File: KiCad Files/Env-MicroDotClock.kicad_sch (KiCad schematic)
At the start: 40 parts, among them IC1 IS31FL3730-QFLS2-TR, IC2 IS31FL3730-QFLS2-TR, IC3 IS31FL3730-QFLS2-TR, IC4 IS31FL3730-QFLS2-TR, M1 LTP-305G, M2 LTP-305G, M3 LTP-305G, M4 LTP-305G, M5 LTP-305G, M6 LTP-305G, M7 LTP-305G, M8 LTP-305G, Q1 2SC1815, SW1 SW_Push, SW2 SW_Push, SW3 SW_Push, SW4 SW_Push, SW5 DIP SPST, U1 Pico, U3 DS3231M

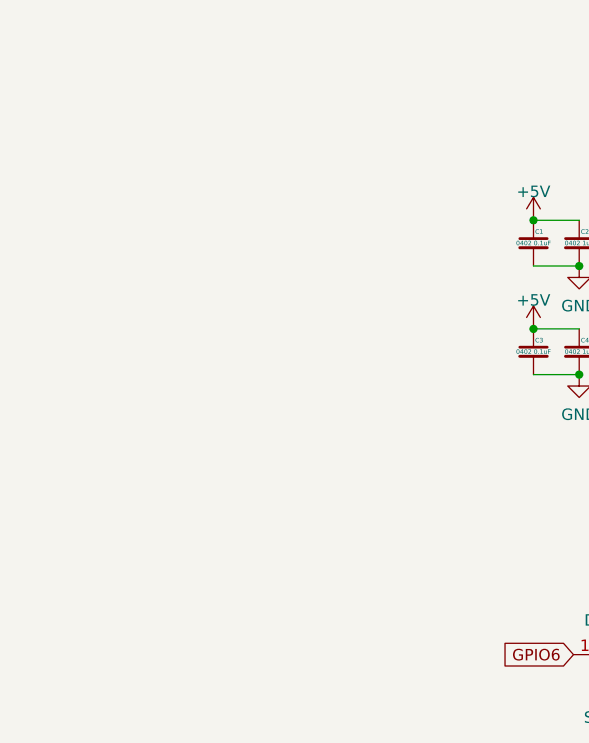
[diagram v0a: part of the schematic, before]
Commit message: dont recall what I changed, probably cleaned some bits up before generating gerber
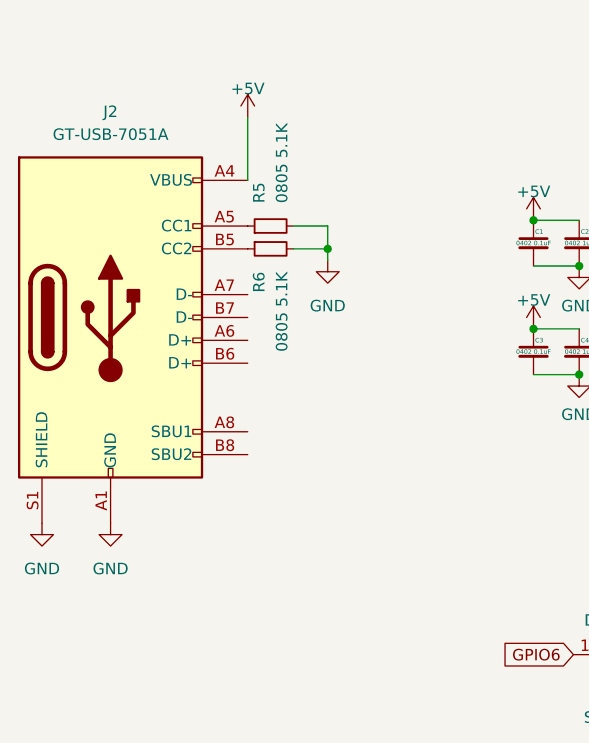
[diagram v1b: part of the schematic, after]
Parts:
- added J2: GT-USB-7051A, Connector_USB:USB_C_Receptacle_G-Switch_GT-USB-7051x, symbol Connector:USB_C_Receptacle_USB2.0
- added R5, R6: 0805 5.1K, Resistor_SMD:R_0805_2012Metric, symbol Device:R_Small
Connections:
- net +5V: now also J2.A4 (VBUS), J2.A9 (VBUS), J2.B4 (VBUS), J2.B9 (VBUS)
- net GND: now also J2.A1 (GND), J2.A12 (GND), J2.B1 (GND), J2.B12 (GND), J2.S1 (SHIELD), R5.2, R6.2
- new net: J2.B5 (CC2), R6.1
- new net: J2.A5 (CC1), R5.1
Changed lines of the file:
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@@
   (junction (at 163.195 168.91) (diameter 0) (color 0 0 0 0)
   )
+  (junction (at -4.445 36.83) (diameter 0) (color 0 0 0 0)
+  )
   (junction (at 170.18 129.54) (diameter 0) (color 0 0 0 0)
   )
@@
     (stroke (width 0) (type default))
   )
+  (wire (pts (xy -4.445 38.1) (xy -4.445 36.83))
+    (stroke (width 0) (type default))
+  )
   (wire (pts (xy 173.355 49.53) (xy 173.355 36.83))
     (stroke (width 0) (type default))
@@
     (stroke (width 0) (type default))
   )
+  (wire (pts (xy -8.255 34.29) (xy -4.445 34.29))
+    (stroke (width 0) (type default))
+  )
   (wire (pts (xy 33.02 81.915) (xy 33.02 94.615))
     (stroke (width 0) (type default))
@@
     (stroke (width 0) (type default))
   )
+  (wire (pts (xy -4.445 34.29) (xy -4.445 36.83))
+    (stroke (width 0) (type default))
+  )
   (wire (pts (xy 33.02 94.615) (xy 33.02 105.41))
     (stroke (width 0) (type default))
@@
     (stroke (width 0) (type default))
   )
+  (wire (pts (xy -13.335 22.225) (xy -13.335 29.21))
+    (stroke (width 0) (type default))
+  )
+  (wire (pts (xy -4.445 36.83) (xy -8.255 36.83))
+    (stroke (width 0) (type default))
+  )
   (wire (pts (xy 99.06 158.75) (xy 99.06 162.56))
     (stroke (width 0) (type default))
@@
     )
   )
+  (symbol (lib_id "Device:R_Small") (at -10.795 36.83 90) (mirror x) (unit 1)
+    (in_bom yes) (on_board yes) (dnp no)
+    (property "Reference" "R6" (at -12.065 39.37 0)
+      (effects (font (size 1.27 1.27)) (justify left))
+    )
+    (property "Value" "0805 5.1K" (at -9.525 39.37 0)
+      (effects (font (size 1.27 1.27)) (justify left))
+    )
+    (property "Footprint" "Resistor_SMD:R_0805_2012Metric" (at -10.795 36.83 0)
+      (effects (font (size 1.27 1.27)) hide)
+    )
+    (property "Datasheet" "~" (at -10.795 36.83 0)
+      (effects (font (size 1.27 1.27)) hide)
+    )
+    (pin "1")
+    (pin "2")
+    (instances
+      (project "Env-MicroDotClock"
+        (path "/3dbeb8d8-208e-4f6d-8d30-b14372f68a4f"
+          (reference "R6") (unit 1)
+        )
+      )
+    )
+  )
   (symbol (lib_id "power:GND") (at 80.645 73.025 0) (mirror y) (unit 1)
     (in_bom yes) (on_board yes) (dnp no) (fields_autoplaced)
@@
     )
   )
+  (symbol (lib_id "Connector:USB_C_Receptacle_USB2.0") (at -28.575 44.45 0) (unit 1)
+    (in_bom yes) (on_board yes) (dnp no) (fields_autoplaced)
+    (property "Reference" "J2" (at -28.575 21.59 0)
+      (effects (font (size 1.27 1.27)))
+    )
+    (property "Value" "GT-USB-7051A" (at -28.575 24.13 0)
+      (effects (font (size 1.27 1.27)))
+    )
+    (property "Footprint" "Connector_USB:USB_C_Receptacle_G-Switch_GT-USB-7051x" (at -24.765 44.45 0)
+      (effects (font (size 1.27 1.27)) hide)
+    )
+    (property "Datasheet" "https://www.usb.org/sites/default/files/documents/usb_type-c.zip" (at -24.765 44.45 0)
+      (effects (font (size 1.27 1.27)) hide)
+    )
+    (pin "A1")
+    (pin "A12")
+    (pin "A4")
+    (pin "A5")
+    (pin "A6")
+    (pin "A7")
+    (pin "A8")
+    (pin "A9")
+    (pin "B1")
+    (pin "B12")
+    (pin "B4")
+    (pin "B5")
+    (pin "B6")
+    (pin "B7")
+    (pin "B8")
+    (pin "B9")
+    (pin "S1")
+    (instances
+      (project "Env-MicroDotClock"
+        (path "/3dbeb8d8-208e-4f6d-8d30-b14372f68a4f"
+          (reference "J2") (unit 1)
+        )
+      )
+    )
+  )
   (symbol (lib_id "Transistor_BJT:BC817") (at 154.305 181.61 0) (unit 1)
     (in_bom yes) (on_board yes) (dnp no) (fields_autoplaced)
@@
     )
   )
+  (symbol (lib_id "power:+5V") (at -13.335 22.225 0) (unit 1)
+    (in_bom yes) (on_board yes) (dnp no) (fields_autoplaced)
+    (property "Reference" "#PWR044" (at -13.335 26.035 0)
+      (effects (font (size 1.27 1.27)) hide)
+    )
+    (property "Value" "+5V" (at -13.335 19.05 0)
+      (effects (font (size 1.27 1.27)))
+    )
+    (property "Footprint" "" (at -13.335 22.225 0)
+      (effects (font (size 1.27 1.27)) hide)
+    )
+    (property "Datasheet" "" (at -13.335 22.225 0)
+      (effects (font (size 1.27 1.27)) hide)
+    )
+    (pin "1")
+    (instances
+      (project "Env-MicroDotClock"
+        (path "/3dbeb8d8-208e-4f6d-8d30-b14372f68a4f"
+          (reference "#PWR044") (unit 1)
+        )
+      )
+    )
+  )
   (symbol (lib_id "ltp-305g:LTP-305G") (at 102.87 104.775 0) (unit 1)
     (in_bom yes) (on_board yes) (dnp no) (fields_autoplaced)
@@
     )
   )
+  (symbol (lib_id "power:GND") (at -28.575 67.31 0) (mirror y) (unit 1)
+    (in_bom yes) (on_board yes) (dnp no) (fields_autoplaced)
+    (property "Reference" "#PWR046" (at -28.575 73.66 0)
+      (effects (font (size 1.27 1.27)) hide)
+    )
+    (property "Value" "GND" (at -28.575 72.39 0)
+      (effects (font (size 1.27 1.27)))
+    )
+    (property "Footprint" "" (at -28.575 67.31 0)
+      (effects (font (size 1.27 1.27)) hide)
+    )
+    (property "Datasheet" "" (at -28.575 67.31 0)
+      (effects (font (size 1.27 1.27)) hide)
+    )
+    (pin "1")
+    (instances
+      (project "Env-MicroDotClock"
+        (path "/3dbeb8d8-208e-4f6d-8d30-b14372f68a4f"
+          (reference "#PWR046") (unit 1)
+        )
+      )
+    )
+  )
   (symbol (lib_id "ltp-305g:LTP-305G") (at 229.87 34.925 0) (unit 1)
     (in_bom yes) (on_board yes) (dnp no) (fields_autoplaced)
@@
     )
   )
+  (symbol (lib_id "Device:R_Small") (at -10.795 34.29 90) (unit 1)
+    (in_bom yes) (on_board yes) (dnp no)
+    (property "Reference" "R5" (at -12.065 31.75 0)
+      (effects (font (size 1.27 1.27)) (justify left))
+    )
+    (property "Value" "0805 5.1K" (at -9.525 31.75 0)
+      (effects (font (size 1.27 1.27)) (justify left))
+    )
+    (property "Footprint" "Resistor_SMD:R_0805_2012Metric" (at -10.795 34.29 0)
+      (effects (font (size 1.27 1.27)) hide)
+    )
+    (property "Datasheet" "~" (at -10.795 34.29 0)
+      (effects (font (size 1.27 1.27)) hide)
+    )
+    (pin "1")
+    (pin "2")
+    (instances
+      (project "Env-MicroDotClock"
+        (path "/3dbeb8d8-208e-4f6d-8d30-b14372f68a4f"
+          (reference "R5") (unit 1)
+        )
+      )
+    )
+  )
   (symbol (lib_id "power:GND") (at 23.495 38.735 0) (unit 1)
     (in_bom yes) (on_board yes) (dnp no) (fields_autoplaced)
@@
     )
   )
+  (symbol (lib_id "power:GND") (at -4.445 38.1 0) (mirror y) (unit 1)
+    (in_bom yes) (on_board yes) (dnp no) (fields_autoplaced)
+    (property "Reference" "#PWR047" (at -4.445 44.45 0)
+      (effects (font (size 1.27 1.27)) hide)
+    )
+    (property "Value" "GND" (at -4.445 43.18 0)
+      (effects (font (size 1.27 1.27)))
+    )
+    (property "Footprint" "" (at -4.445 38.1 0)
+      (effects (font (size 1.27 1.27)) hide)
+    )
+    (property "Datasheet" "" (at -4.445 38.1 0)
+      (effects (font (size 1.27 1.27)) hide)
+    )
+    (pin "1")
+    (instances
+      (project "Env-MicroDotClock"
+        (path "/3dbeb8d8-208e-4f6d-8d30-b14372f68a4f"
+          (reference "#PWR047") (unit 1)
+        )
+      )
+    )
+  )
   (symbol (lib_id "power:+5V") (at 18.415 33.655 0) (unit 1)
     (in_bom yes) (on_board yes) (dnp no) (fields_autoplaced)
@@
         )
       )
+    )
+  )
+  (symbol (lib_id "power:GND") (at -36.195 67.31 0) (mirror y) (unit 1)
+    (in_bom yes) (on_board yes) (dnp no) (fields_autoplaced)
+    (property "Reference" "#PWR045" (at -36.195 73.66 0)
+      (effects (font (size 1.27 1.27)) hide)
+    )
+    (property "Value" "GND" (at -36.195 72.39 0)
+      (effects (font (size 1.27 1.27)))
+    )
+    (property "Footprint" "" (at -36.195 67.31 0)
+      (effects (font (size 1.27 1.27)) hide)
+    )
+    (property "Datasheet" "" (at -36.195 67.31 0)
+      (effects (font (size 1.27 1.27)) hide)
+    )
+    (pin "1")
+    (instances
+      (project "Env-MicroDotClock"
+        (path "/3dbeb8d8-208e-4f6d-8d30-b14372f68a4f"
+          (reference "#PWR045") (unit 1)
+        )
+      )

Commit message: updated to reflect current vision.
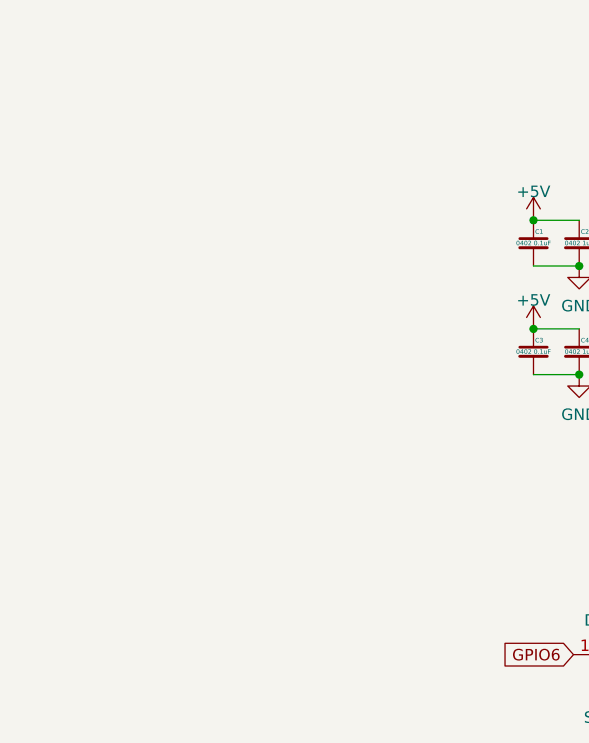
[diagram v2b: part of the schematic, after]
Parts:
- removed J2: GT-USB-7051A, Connector_USB:USB_C_Receptacle_G-Switch_GT-USB-7051x, symbol Connector:USB_C_Receptacle_USB2.0
- removed R5, R6: 0805 5.1K, Resistor_SMD:R_0805_2012Metric, symbol Device:R_Small
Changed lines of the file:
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@@
   (junction (at 163.195 168.91) (diameter 0) (color 0 0 0 0)
   )
-  (junction (at -4.445 36.83) (diameter 0) (color 0 0 0 0)
-  )
   (junction (at 170.18 129.54) (diameter 0) (color 0 0 0 0)
   )
@@
     (stroke (width 0) (type default))
   )
-  (wire (pts (xy -4.445 38.1) (xy -4.445 36.83))
-    (stroke (width 0) (type default))
-  )
   (wire (pts (xy 173.355 49.53) (xy 173.355 36.83))
     (stroke (width 0) (type default))
@@
     (stroke (width 0) (type default))
   )
-  (wire (pts (xy -8.255 34.29) (xy -4.445 34.29))
-    (stroke (width 0) (type default))
-  )
   (wire (pts (xy 33.02 81.915) (xy 33.02 94.615))
     (stroke (width 0) (type default))
@@
     (stroke (width 0) (type default))
   )
-  (wire (pts (xy -4.445 34.29) (xy -4.445 36.83))
-    (stroke (width 0) (type default))
-  )
   (wire (pts (xy 33.02 94.615) (xy 33.02 105.41))
     (stroke (width 0) (type default))
@@
     (stroke (width 0) (type default))
   )
-  (wire (pts (xy -13.335 22.225) (xy -13.335 29.21))
-    (stroke (width 0) (type default))
-  )
-  (wire (pts (xy -4.445 36.83) (xy -8.255 36.83))
-    (stroke (width 0) (type default))
-  )
   (wire (pts (xy 99.06 158.75) (xy 99.06 162.56))
     (stroke (width 0) (type default))
@@
     )
   )
-  (symbol (lib_id "Device:R_Small") (at -10.795 36.83 90) (mirror x) (unit 1)
-    (in_bom yes) (on_board yes) (dnp no)
-    (property "Reference" "R6" (at -12.065 39.37 0)
-      (effects (font (size 1.27 1.27)) (justify left))
-    )
-    (property "Value" "0805 5.1K" (at -9.525 39.37 0)
-      (effects (font (size 1.27 1.27)) (justify left))
-    )
-    (property "Footprint" "Resistor_SMD:R_0805_2012Metric" (at -10.795 36.83 0)
-      (effects (font (size 1.27 1.27)) hide)
-    )
-    (property "Datasheet" "~" (at -10.795 36.83 0)
-      (effects (font (size 1.27 1.27)) hide)
-    )
-    (pin "1")
-    (pin "2")
-    (instances
-      (project "Env-MicroDotClock"
-        (path "/3dbeb8d8-208e-4f6d-8d30-b14372f68a4f"
-          (reference "R6") (unit 1)
-        )
-      )
-    )
-  )
   (symbol (lib_id "power:GND") (at 80.645 73.025 0) (mirror y) (unit 1)
     (in_bom yes) (on_board yes) (dnp no) (fields_autoplaced)
@@
     )
   )
-  (symbol (lib_id "Connector:USB_C_Receptacle_USB2.0") (at -28.575 44.45 0) (unit 1)
-    (in_bom yes) (on_board yes) (dnp no) (fields_autoplaced)
-    (property "Reference" "J2" (at -28.575 21.59 0)
-      (effects (font (size 1.27 1.27)))
-    )
-    (property "Value" "GT-USB-7051A" (at -28.575 24.13 0)
-      (effects (font (size 1.27 1.27)))
-    )
-    (property "Footprint" "Connector_USB:USB_C_Receptacle_G-Switch_GT-USB-7051x" (at -24.765 44.45 0)
-      (effects (font (size 1.27 1.27)) hide)
-    )
-    (property "Datasheet" "https://www.usb.org/sites/default/files/documents/usb_type-c.zip" (at -24.765 44.45 0)
-      (effects (font (size 1.27 1.27)) hide)
-    )
-    (pin "A1")
-    (pin "A12")
-    (pin "A4")
-    (pin "A5")
-    (pin "A6")
-    (pin "A7")
-    (pin "A8")
-    (pin "A9")
-    (pin "B1")
-    (pin "B12")
-    (pin "B4")
-    (pin "B5")
-    (pin "B6")
-    (pin "B7")
-    (pin "B8")
-    (pin "B9")
-    (pin "S1")
-    (instances
-      (project "Env-MicroDotClock"
-        (path "/3dbeb8d8-208e-4f6d-8d30-b14372f68a4f"
-          (reference "J2") (unit 1)
-        )
-      )
-    )
-  )
   (symbol (lib_id "Transistor_BJT:BC817") (at 154.305 181.61 0) (unit 1)
     (in_bom yes) (on_board yes) (dnp no) (fields_autoplaced)
@@
     )
   )
-  (symbol (lib_id "power:+5V") (at -13.335 22.225 0) (unit 1)
-    (in_bom yes) (on_board yes) (dnp no) (fields_autoplaced)
-    (property "Reference" "#PWR044" (at -13.335 26.035 0)
-      (effects (font (size 1.27 1.27)) hide)
-    )
-    (property "Value" "+5V" (at -13.335 19.05 0)
-      (effects (font (size 1.27 1.27)))
-    )
-    (property "Footprint" "" (at -13.335 22.225 0)
-      (effects (font (size 1.27 1.27)) hide)
-    )
-    (property "Datasheet" "" (at -13.335 22.225 0)
-      (effects (font (size 1.27 1.27)) hide)
-    )
-    (pin "1")
-    (instances
-      (project "Env-MicroDotClock"
-        (path "/3dbeb8d8-208e-4f6d-8d30-b14372f68a4f"
-          (reference "#PWR044") (unit 1)
-        )
-      )
-    )
-  )
   (symbol (lib_id "ltp-305g:LTP-305G") (at 102.87 104.775 0) (unit 1)
     (in_bom yes) (on_board yes) (dnp no) (fields_autoplaced)
@@
     )
   )
-  (symbol (lib_id "power:GND") (at -28.575 67.31 0) (mirror y) (unit 1)
-    (in_bom yes) (on_board yes) (dnp no) (fields_autoplaced)
-    (property "Reference" "#PWR046" (at -28.575 73.66 0)
-      (effects (font (size 1.27 1.27)) hide)
-    )
-    (property "Value" "GND" (at -28.575 72.39 0)
-      (effects (font (size 1.27 1.27)))
-    )
-    (property "Footprint" "" (at -28.575 67.31 0)
-      (effects (font (size 1.27 1.27)) hide)
-    )
-    (property "Datasheet" "" (at -28.575 67.31 0)
-      (effects (font (size 1.27 1.27)) hide)
-    )
-    (pin "1")
-    (instances
-      (project "Env-MicroDotClock"
-        (path "/3dbeb8d8-208e-4f6d-8d30-b14372f68a4f"
-          (reference "#PWR046") (unit 1)
-        )
-      )
-    )
-  )
   (symbol (lib_id "ltp-305g:LTP-305G") (at 229.87 34.925 0) (unit 1)
     (in_bom yes) (on_board yes) (dnp no) (fields_autoplaced)
@@
     )
   )
-  (symbol (lib_id "Device:R_Small") (at -10.795 34.29 90) (unit 1)
-    (in_bom yes) (on_board yes) (dnp no)
-    (property "Reference" "R5" (at -12.065 31.75 0)
-      (effects (font (size 1.27 1.27)) (justify left))
-    )
-    (property "Value" "0805 5.1K" (at -9.525 31.75 0)
-      (effects (font (size 1.27 1.27)) (justify left))
-    )
-    (property "Footprint" "Resistor_SMD:R_0805_2012Metric" (at -10.795 34.29 0)
-      (effects (font (size 1.27 1.27)) hide)
-    )
-    (property "Datasheet" "~" (at -10.795 34.29 0)
-      (effects (font (size 1.27 1.27)) hide)
-    )
-    (pin "1")
-    (pin "2")
-    (instances
-      (project "Env-MicroDotClock"
-        (path "/3dbeb8d8-208e-4f6d-8d30-b14372f68a4f"
-          (reference "R5") (unit 1)
-        )
-      )
-    )
-  )
   (symbol (lib_id "power:GND") (at 23.495 38.735 0) (unit 1)
     (in_bom yes) (on_board yes) (dnp no) (fields_autoplaced)
@@
     )
   )
-  (symbol (lib_id "power:GND") (at -4.445 38.1 0) (mirror y) (unit 1)
-    (in_bom yes) (on_board yes) (dnp no) (fields_autoplaced)
-    (property "Reference" "#PWR047" (at -4.445 44.45 0)
-      (effects (font (size 1.27 1.27)) hide)
-    )
-    (property "Value" "GND" (at -4.445 43.18 0)
-      (effects (font (size 1.27 1.27)))
-    )
-    (property "Footprint" "" (at -4.445 38.1 0)
-      (effects (font (size 1.27 1.27)) hide)
-    )
-    (property "Datasheet" "" (at -4.445 38.1 0)
-      (effects (font (size 1.27 1.27)) hide)
-    )
-    (pin "1")
-    (instances
-      (project "Env-MicroDotClock"
-        (path "/3dbeb8d8-208e-4f6d-8d30-b14372f68a4f"
-          (reference "#PWR047") (unit 1)
-        )
-      )
-    )
-  )
   (symbol (lib_id "power:+5V") (at 18.415 33.655 0) (unit 1)
     (in_bom yes) (on_board yes) (dnp no) (fields_autoplaced)
@@
         )
       )
-    )
-  )
-  (symbol (lib_id "power:GND") (at -36.195 67.31 0) (mirror y) (unit 1)
-    (in_bom yes) (on_board yes) (dnp no) (fields_autoplaced)
-    (property "Reference" "#PWR045" (at -36.195 73.66 0)
-      (effects (font (size 1.27 1.27)) hide)
-    )
-    (property "Value" "GND" (at -36.195 72.39 0)
-      (effects (font (size 1.27 1.27)))
-    )
-    (property "Footprint" "" (at -36.195 67.31 0)
-      (effects (font (size 1.27 1.27)) hide)
-    )
-    (property "Datasheet" "" (at -36.195 67.31 0)
-      (effects (font (size 1.27 1.27)) hide)
-    )
-    (pin "1")
-    (instances
-      (project "Env-MicroDotClock"
-        (path "/3dbeb8d8-208e-4f6d-8d30-b14372f68a4f"
-          (reference "#PWR045") (unit 1)
-        )
-      )
